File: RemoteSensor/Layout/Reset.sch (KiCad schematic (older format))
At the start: 7 parts, among them Q2 2N7002, SW1 BTN_RST, U6 74LVC2G02

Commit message: Update sensor schematic
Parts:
- Q2: symbol dk_Transistors-FETs-MOSFETs-Single:2N7002 -> RemoteSensor-rescue:2N7002-dk_Transistors-FETs-MOSFETs-Single
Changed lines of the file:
@@
 EESchema Schematic File Version 4
-LIBS:RemoteSensor-cache
-EELAYER 29 0
+EELAYER 30 0
 EELAYER END
 $Descr A4 11693 8268
@@
 $EndComp
 $Comp
-L SparkFun-PowerSymbols:GND #GND?
+L RemoteSensor-rescue:GND-SparkFun-PowerSymbols #GND?
 U 1 1 5EF5A921
 P 5650 4150
@@
 $EndComp
 $Comp
-L SparkFun-PowerSymbols:GND #GND?
+L RemoteSensor-rescue:GND-SparkFun-PowerSymbols #GND?
 U 1 1 5EF5A935
 P 4800 4100
@@
 	5350 4950 5350 4900
 $Comp
-L dk_Transistors-FETs-MOSFETs-Single:2N7002 Q?
+L RemoteSensor-rescue:2N7002-dk_Transistors-FETs-MOSFETs-Single Q?
 U 1 1 5EF5A94D
 P 6500 3950
@@
 	6500 3750 6500 3450
 $Comp
-L SparkFun-PowerSymbols:3.3V #SUPPLY?
+L RemoteSensor-rescue:3.3V-SparkFun-PowerSymbols #SUPPLY?
 U 1 1 5EF5A963
 P 4800 3650
@@
 $EndComp
 $Comp
-L SparkFun-PowerSymbols:3.3V #SUPPLY?
+L RemoteSensor-rescue:3.3V-SparkFun-PowerSymbols #SUPPLY?
 U 1 1 5EF5A969
 P 5650 3700
@@
 	4350 4950 4950 4950
 $Comp
-L SparkFun-PowerSymbols:GND #GND?
+L RemoteSensor-rescue:GND-SparkFun-PowerSymbols #GND?
 U 1 1 5EF5A98A
 P 5350 4950
@@
 $EndComp
 $Comp
-L SparkFun-PowerSymbols:GND #GND?
+L RemoteSensor-rescue:GND-SparkFun-PowerSymbols #GND?
 U 1 1 5EF5D1D7
 P 5900 2050

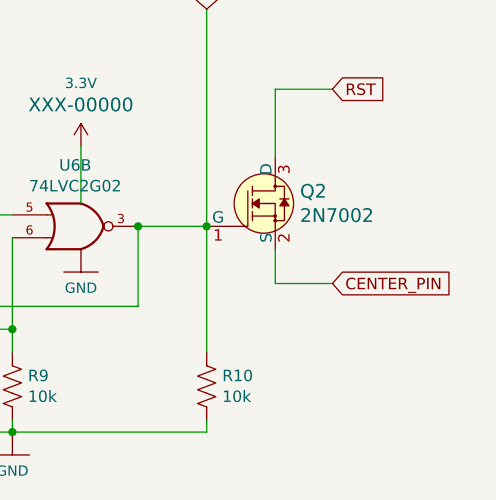
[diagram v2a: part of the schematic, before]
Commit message: Edit layout
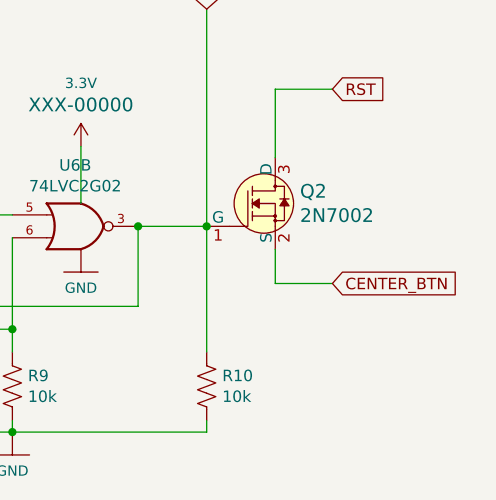
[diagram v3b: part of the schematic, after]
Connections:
- net CENTER_PIN renamed CENTER_BTN
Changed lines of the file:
@@
 RST
 Text GLabel 6750 4300 2    50   Input ~ 0
-CENTER_PIN
+CENTER_BTN
 Text GLabel 3950 3950 0    50   Input ~ 0
 SLEEP_PIN

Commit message: Change what pins are used for i2c
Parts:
- R10, R7, R8, R9: symbol Device:R_US -> RemoteSensor-rescue:R_US-Device
- SW1: symbol Switch:SW_Push -> RemoteSensor-rescue:SW_Push-Switch
- U6: symbol 74xGxx:74LVC2G02 -> RemoteSensor-rescue:74LVC2G02-74xGxx
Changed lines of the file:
@@
 $EndDescr
 $Comp
-L Device:R_US R?
+L RemoteSensor-rescue:R_US-Device R?
 U 1 1 5EF5A915
 P 5350 4750
@@
 $EndComp
 $Comp
-L Device:R_US R?
+L RemoteSensor-rescue:R_US-Device R?
 U 1 1 5EF5A91B
 P 4350 4750
@@
 $EndComp
 $Comp
-L 74xGxx:74LVC2G02 U?
+L RemoteSensor-rescue:74LVC2G02-74xGxx U?
 U 2 1 5EF5A927
 P 5650 4050
@@
 	4800 3900 4800 3650
 $Comp
-L 74xGxx:74LVC2G02 U?
+L RemoteSensor-rescue:74LVC2G02-74xGxx U?
 U 1 1 5EF5A92F
 P 4800 4000
@@
 $EndComp
 $Comp
-L Device:R_US R?
+L RemoteSensor-rescue:R_US-Device R?
 U 1 1 5EF5A953
 P 6200 4750
@@
 	6200 4050 6200 3100
 $Comp
-L Device:R_US R?
+L RemoteSensor-rescue:R_US-Device R?
 U 1 1 5EF5A980
 P 4950 4750
@@
 Connection ~ 5050 4000
 $Comp
-L Switch:SW_Push SW?
+L RemoteSensor-rescue:SW_Push-Switch SW?
 U 1 1 5EF5D1D1
 P 5550 2050

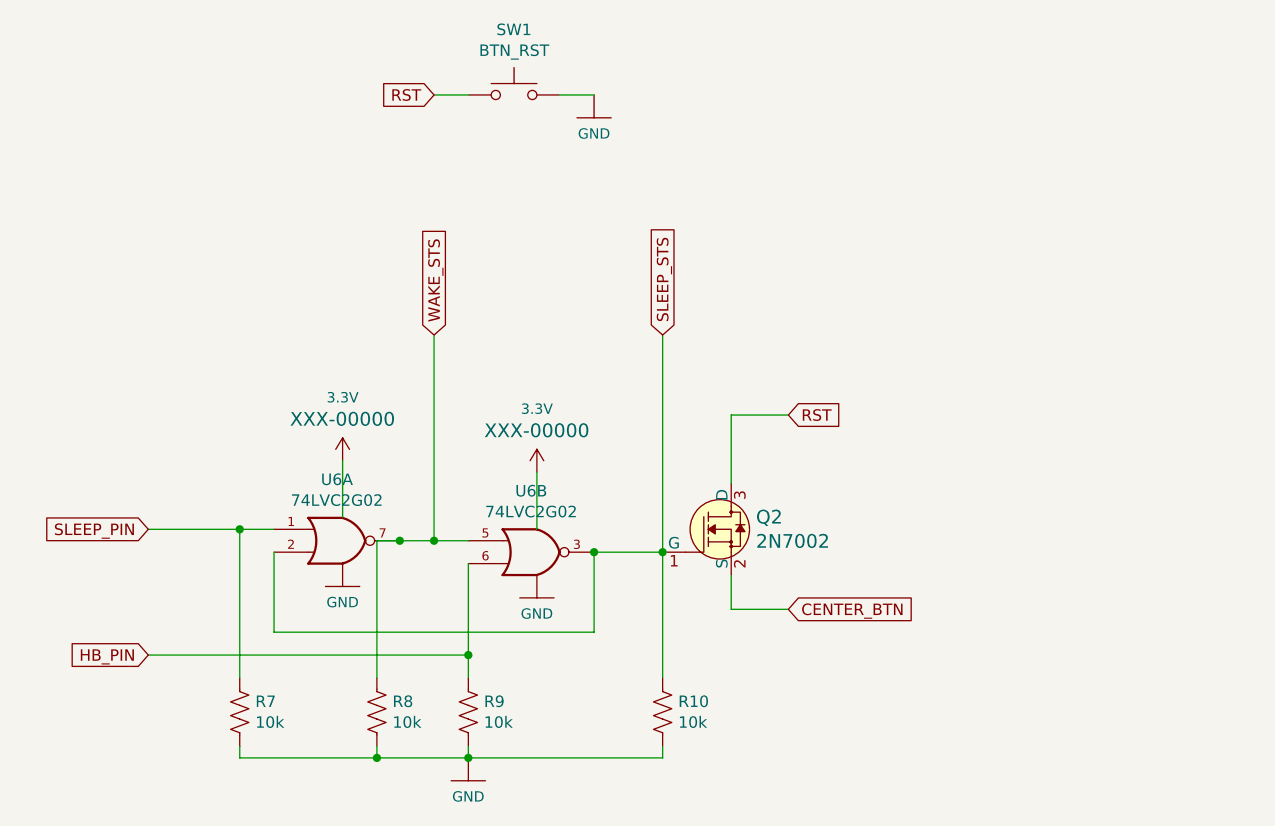
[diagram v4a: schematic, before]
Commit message: Another layout
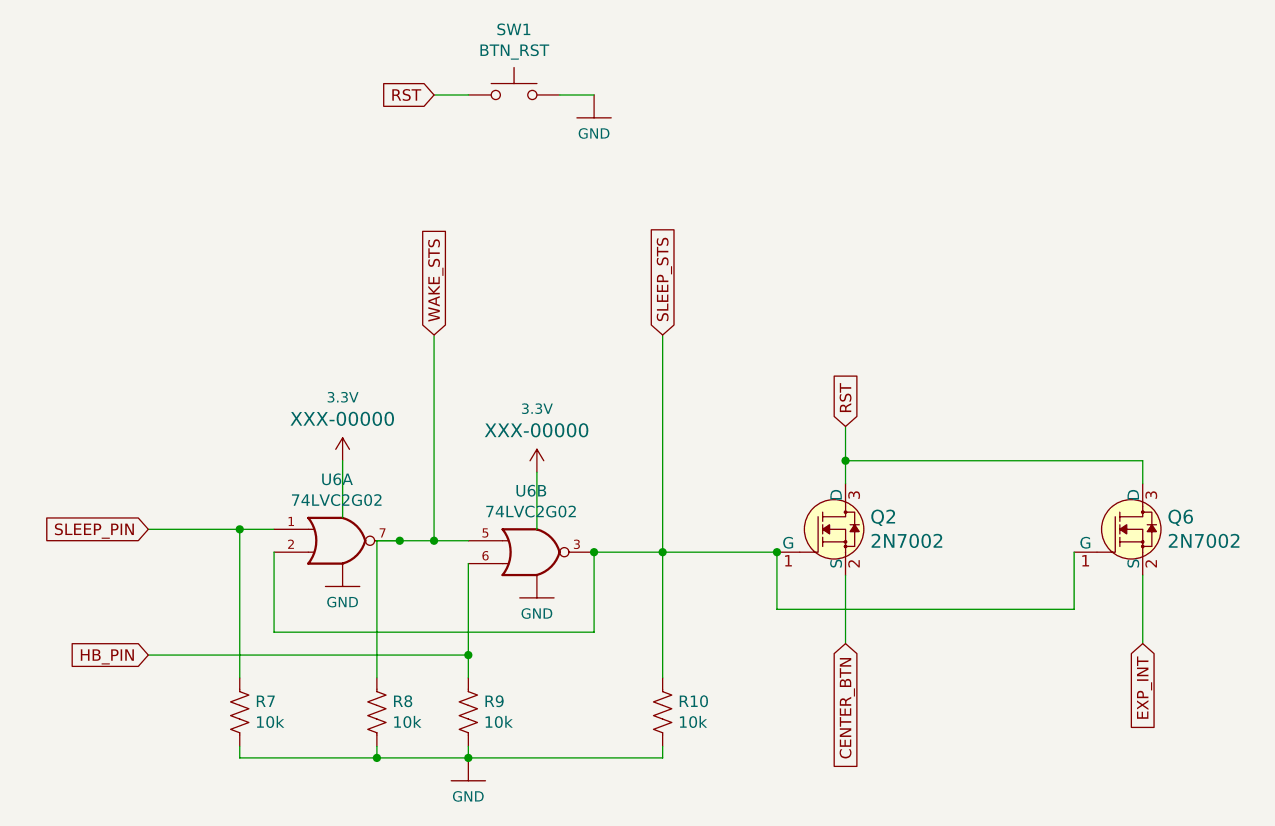
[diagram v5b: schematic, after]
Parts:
- added Q6: 2N7002, digikey-footprints:SOT-23-3, symbol RemoteSensor-rescue:2N7002-dk_Transistors-FETs-MOSFETs-Single
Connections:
- net RST: now also Q6.3 (D)
- net SLEEP_STS: now also Q6.1 (G)
- new net EXP_INT: Q6.2 (S)
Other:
- moved on the sheet: Q2
